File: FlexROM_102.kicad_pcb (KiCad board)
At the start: 2 copper layers, 16.5 x 34.3 mm, 7 parts, among them J1 27C256 DIP LEGS, U1 28C256

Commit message: kicad 6
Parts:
- JP1: value ~CS~ breakout (REX TP1) -> ~{CS} breakout (REX TP1)
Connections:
- net /A14_~WE renamed /A14_~{WE}
- net /~CS_IN renamed /~{CS_IN}
- net /~CS_OUT renamed /~{CS_OUT}
- net /~OE renamed /~{OE}
- net /~WE renamed /~{WE}
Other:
- net class Default removed
- board text added: "REX main rom: ~{CS} OUT to REX TP1 No REX: ~{CS} OUT to ~{CS} IN"
- board text added: "~{CS} (to REX)"
- board text removed: "REX main rom: ~CS~ OUT to REX TP1 No REX: ~CS~ OUT to ~CS~ IN"
- board text removed: "~CS~ (to REX)"

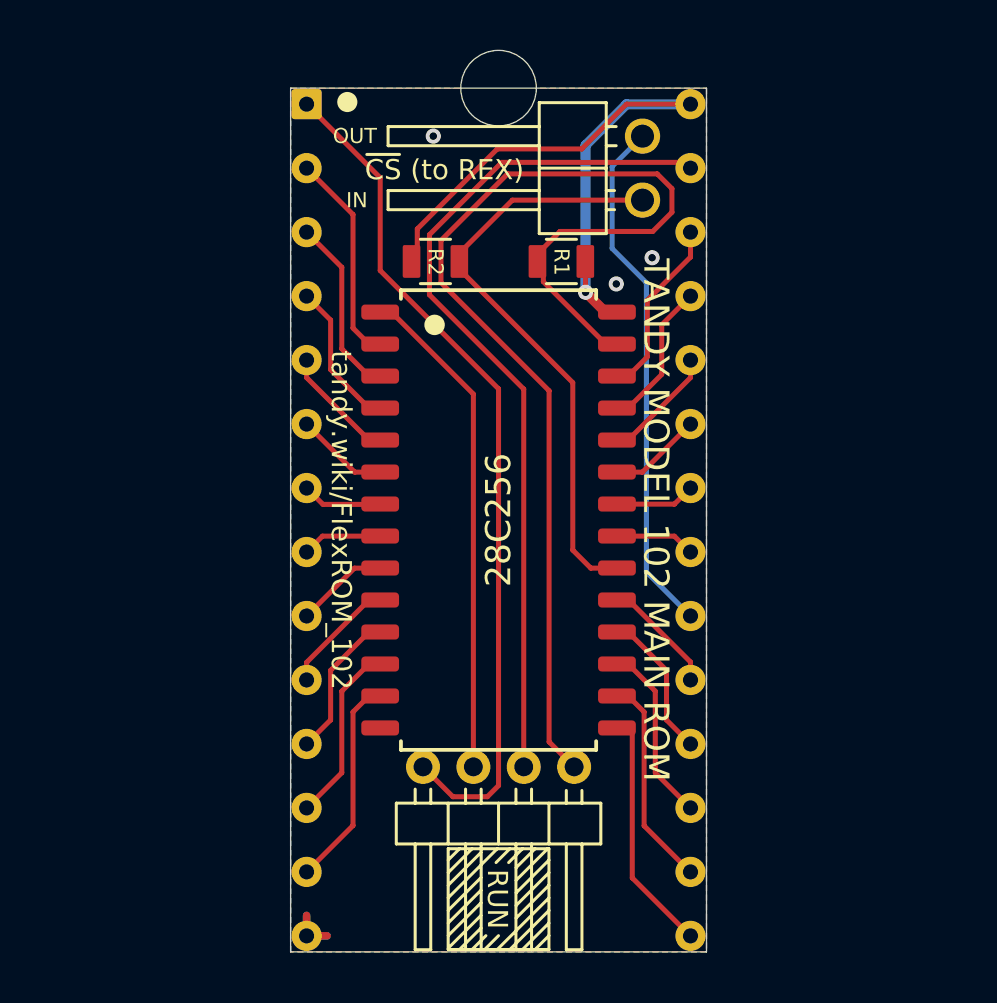
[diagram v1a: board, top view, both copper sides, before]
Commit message: FlexROM_102 outline, sch
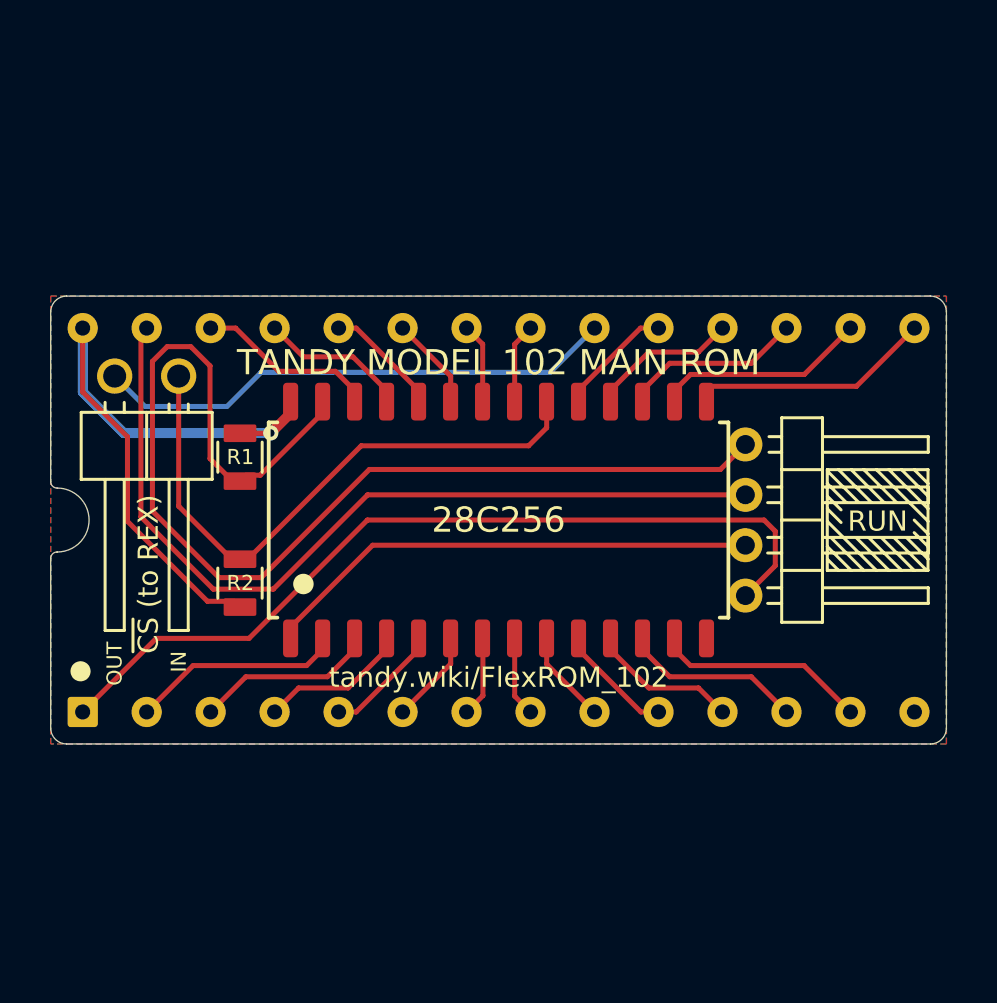
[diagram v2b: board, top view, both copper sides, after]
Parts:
- removed REF**: NPTH_3mm, 000_LOCAL:NPTH_3mm
- J1: footprint 000_LOCAL:DIP28_0.6_pcb_sil_pins -> 000_LOCAL:DIP28_0.6_pcb
- moved JP1 19.7 mm to (114.3, 95.9), turned to -90 degrees
- moved R2 14.9 mm to (116.7, 104.1), turned to -90 degrees
- moved R1 14.9 mm to (116.7, 99.1), turned to -90 degrees
- moved JP2 14.5 mm to (136.8, 98.6), turned to 0 degrees
- turned J1 to 90 degrees
- turned U1 to 90 degrees
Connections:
- net /GND renamed GND
- net /VCC renamed VCC
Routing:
- net GND: track 3.25 -> 0.00 mm, vias 3 -> 0
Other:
- board size 16.5 x 34.3 mm -> 35.6 x 17.8 mm
